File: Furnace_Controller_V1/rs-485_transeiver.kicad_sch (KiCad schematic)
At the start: 18 parts, among them U3 THVD2450DR

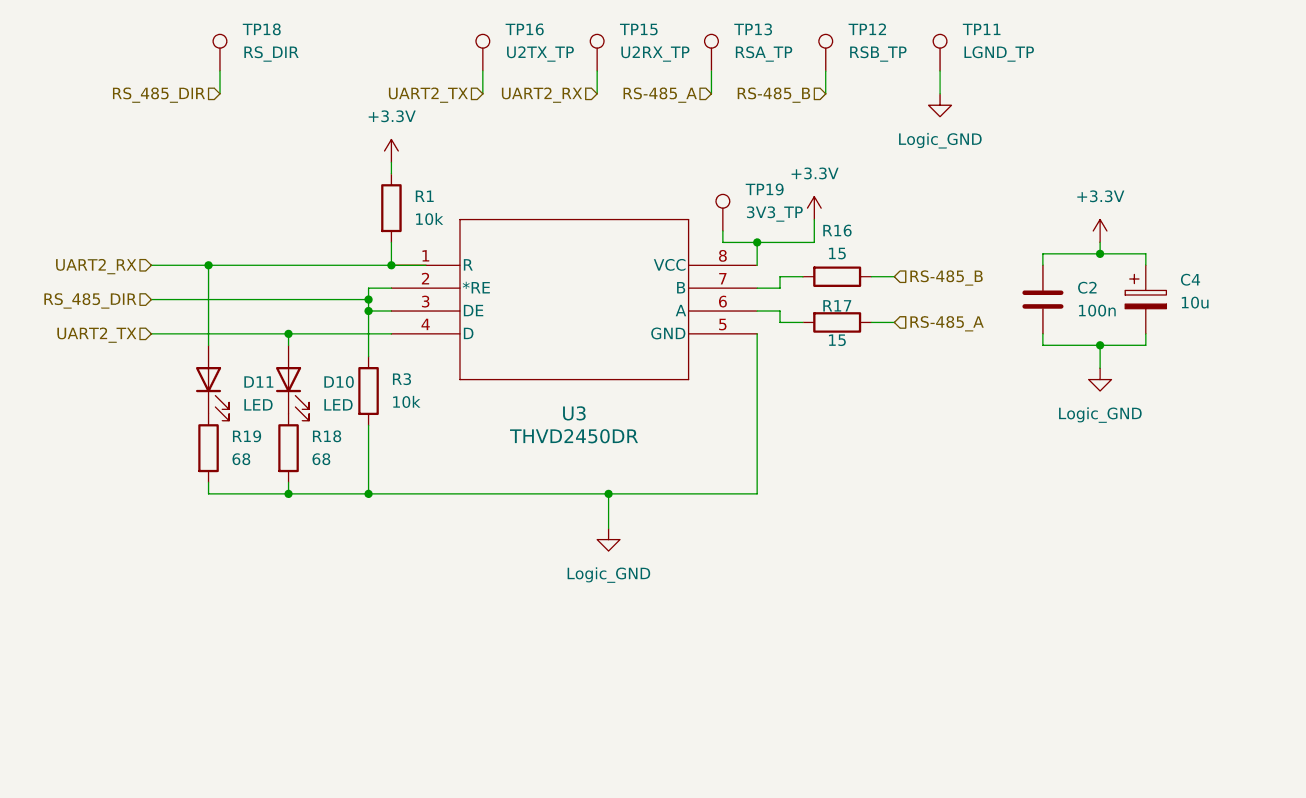
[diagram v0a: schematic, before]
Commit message: V2 dev
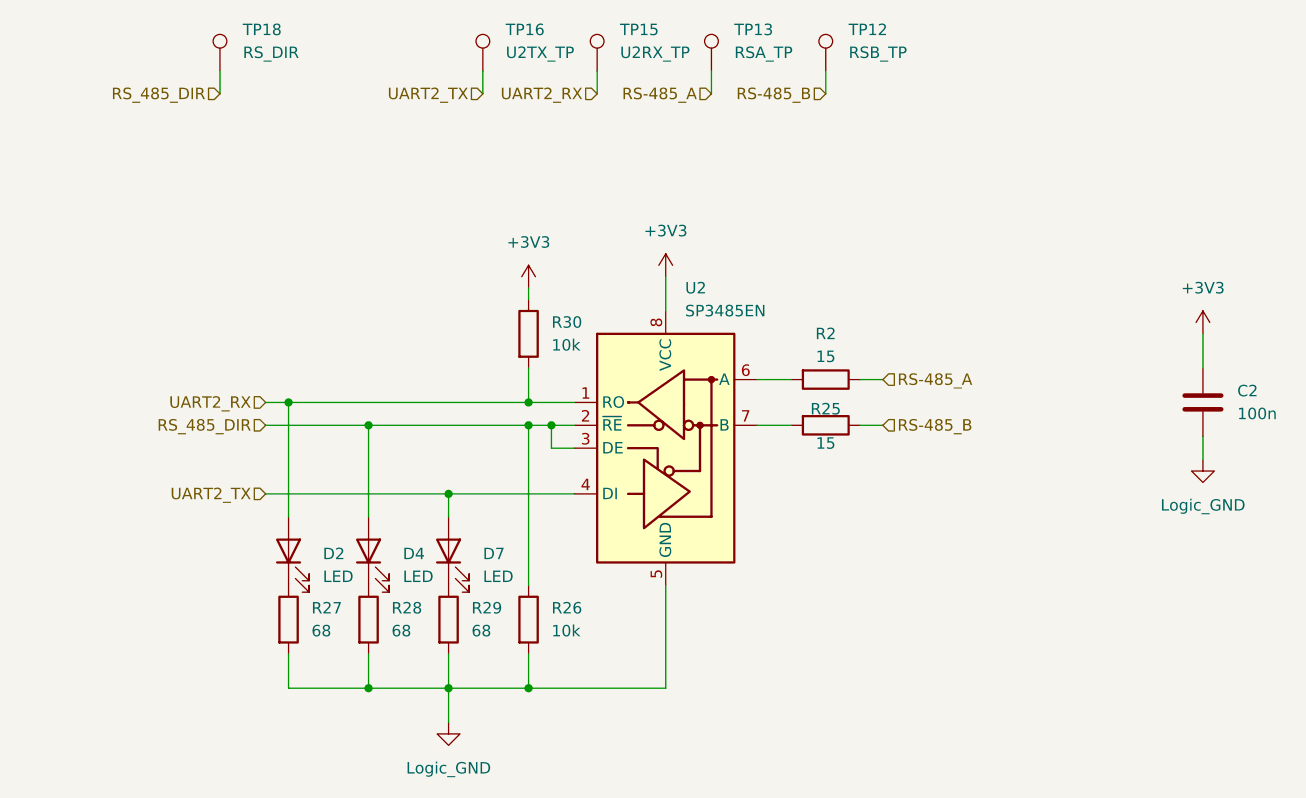
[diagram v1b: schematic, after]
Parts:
- removed C4: 10u, Capacitor_THT:CP_Radial_D5.0mm_P2.00mm, symbol Device:C_Polarized
- removed D10, D11: LED, LED_SMD:LED_0805_2012Metric, symbol Device:LED
- removed R1, R3: 10k, Resistor_SMD:R_0805_2012Metric_Pad1.20x1.40mm_HandSolder, symbol Device:R
- removed R16, R17: 15, Resistor_SMD:R_0805_2012Metric_Pad1.20x1.40mm_HandSolder, symbol Device:R
- removed R18, R19: 68, Resistor_SMD:R_0805_2012Metric_Pad1.20x1.40mm_HandSolder, symbol Device:R
- removed TP11: LGND_TP, TestPoint:TestPoint_Pad_D1.5mm, symbol Connector:TestPoint
- removed TP19: 3V3_TP, TestPoint:TestPoint_Pad_D1.5mm, symbol Connector:TestPoint
- removed U3: THVD2450DR, THVD:SOIC127P600X175-8N, symbol 2026-02-03_10-18-10:THVD2450DR
- added D2, D4, D7: LED, LED_SMD:LED_0603_1608Metric, symbol Device:LED
- added R2, R25: 15, Resistor_SMD:R_0603_1608Metric, symbol Device:R
- added R26, R30: 10k, Resistor_SMD:R_0603_1608Metric, symbol Device:R
- added R27, R28, R29: 68, Resistor_SMD:R_0603_1608Metric, symbol Device:R
- added U2: SP3485EN, Package_SO:SOIC-8_3.9x4.9mm_P1.27mm, symbol Interface_UART:SP3485EN
- C2: footprint Capacitor_SMD:C_0805_2012Metric_Pad1.18x1.45mm_HandSolder -> Capacitor_SMD:C_0603_1608Metric
- TP12, TP13, TP15, TP16, TP18: footprint TestPoint:TestPoint_Pad_D1.5mm -> TestPoint:TestPoint_Pad_D1.0mm
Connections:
- net Logic_GND: now also R26.2, R27.2, R28.2, R29.2, U2.5 (GND)
- net RS-485_A: now also R2.1
- net RS-485_B: now also R25.1
- net RS_485_DIR: now also D4.2 (A), R26.1, U2.2 (~{RE}), U2.3 (DE)
- net UART2_RX: now also D2.2 (A), R30.2, U2.1 (RO)
- net UART2_TX: now also D7.2 (A), U2.4 (DI)
- net +3.3V renamed +3V3
- net +3V3: now also R30.1, U2.8 (VCC)
- new net: D7.1 (K), R29.1
- new net: D2.1 (K), R27.1
- new net: R25.2, U2.7 (B)
- new net: D4.1 (K), R28.1
- new net: R2.2, U2.6 (A)
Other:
- moved on the sheet: C2
